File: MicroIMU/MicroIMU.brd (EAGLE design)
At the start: 7.6 x 19.1 mm, 18 parts, among them IC1 LSM303DLHC

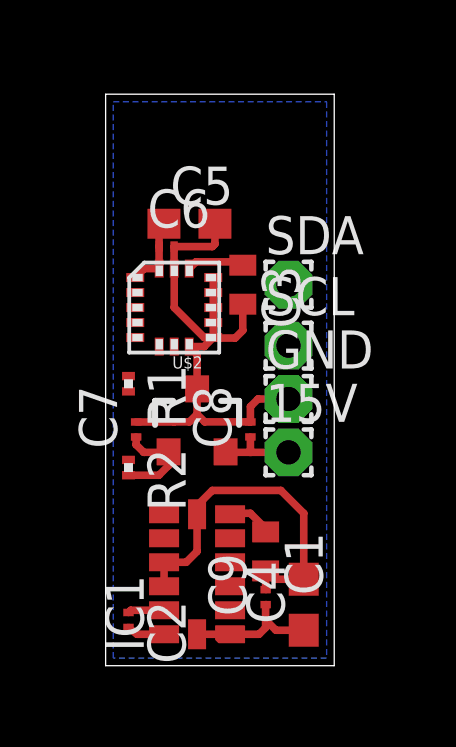
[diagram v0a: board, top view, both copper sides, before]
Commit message: Done routing
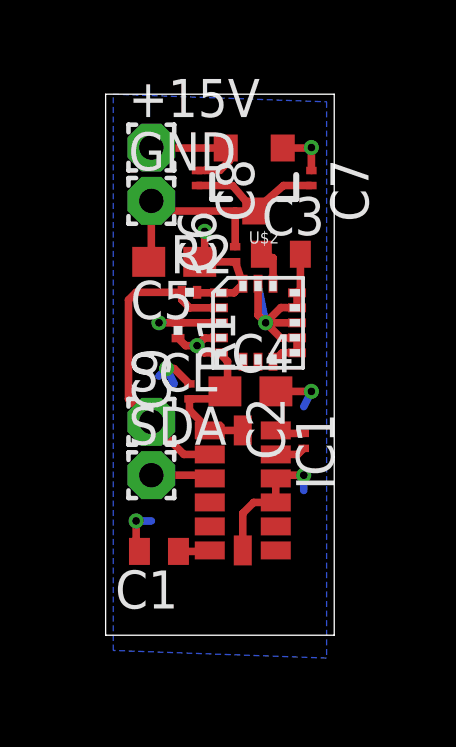
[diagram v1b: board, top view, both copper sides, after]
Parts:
- removed 15V: 15V, wirepad:1,6/0,8
- added +15V: 15V, wirepad:1,6/0,8
- moved C7 10.2 mm to (6.86, 16.3), turned to 270 degrees
- moved C8 8.57 mm to (3.05, 16.3), turned to 270 degrees
- moved C2 8.35 mm to (6.60, 7.49), turned to 90 degrees
- moved U$2 8.35 mm to (4.95, 16.3), turned to 180 degrees
- moved GND 8.03 mm to (1.52, 15.5)
- moved SDA 7.82 mm to (1.52, 6.35)
- moved C4 7.33 mm to (4.83, 9.14), turned to 0 degrees
- moved C9 7.31 mm to (2.79, 9.14)
- moved R2 6.19 mm to (2.79, 12.4), turned to 0 degrees
- moved SCL 5.23 mm to (1.52, 8.13)
- moved C1 3.56 mm to (1.78, 3.81), turned to 180 degrees
- moved IC1 3.18 mm to (4.57, 5.84), turned to 270 degrees
- moved U$1 2.84 mm to (5.08, 11.4)
- moved R1 2.43 mm to (2.41, 11.2)
- moved C6 2.30 mm to (4.32, 13.7), turned to 90 degrees
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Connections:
- net +15V: now also +15V.1; no longer 15V.1
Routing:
- net SDA: track 0.00 -> 14.7 mm, vias 0 -> 1
- net SCL: track 0.00 -> 10.3 mm
- net +3V3: track 10.4 -> 15.7 mm, vias 0 -> 3
- net +15V: track 2.06 -> 4.14 mm
- net N$9: track 1.93 -> 1.27 mm
- net GND: track 31.0 -> 30.8 mm, vias 0 -> 5
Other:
- board size 7.6 x 19.1 mm -> 7.6 x 18 mm
